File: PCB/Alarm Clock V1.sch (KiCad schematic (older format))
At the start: 23 parts, among them P1 CONN_01X02, P4 CONN_02X25, P5 CONN_02X25, SW1 SW_PUSH, SW2 SW_PUSH, SW3 SW_PUSH, SW4 SW_PUSH, SW5 SW_PUSH

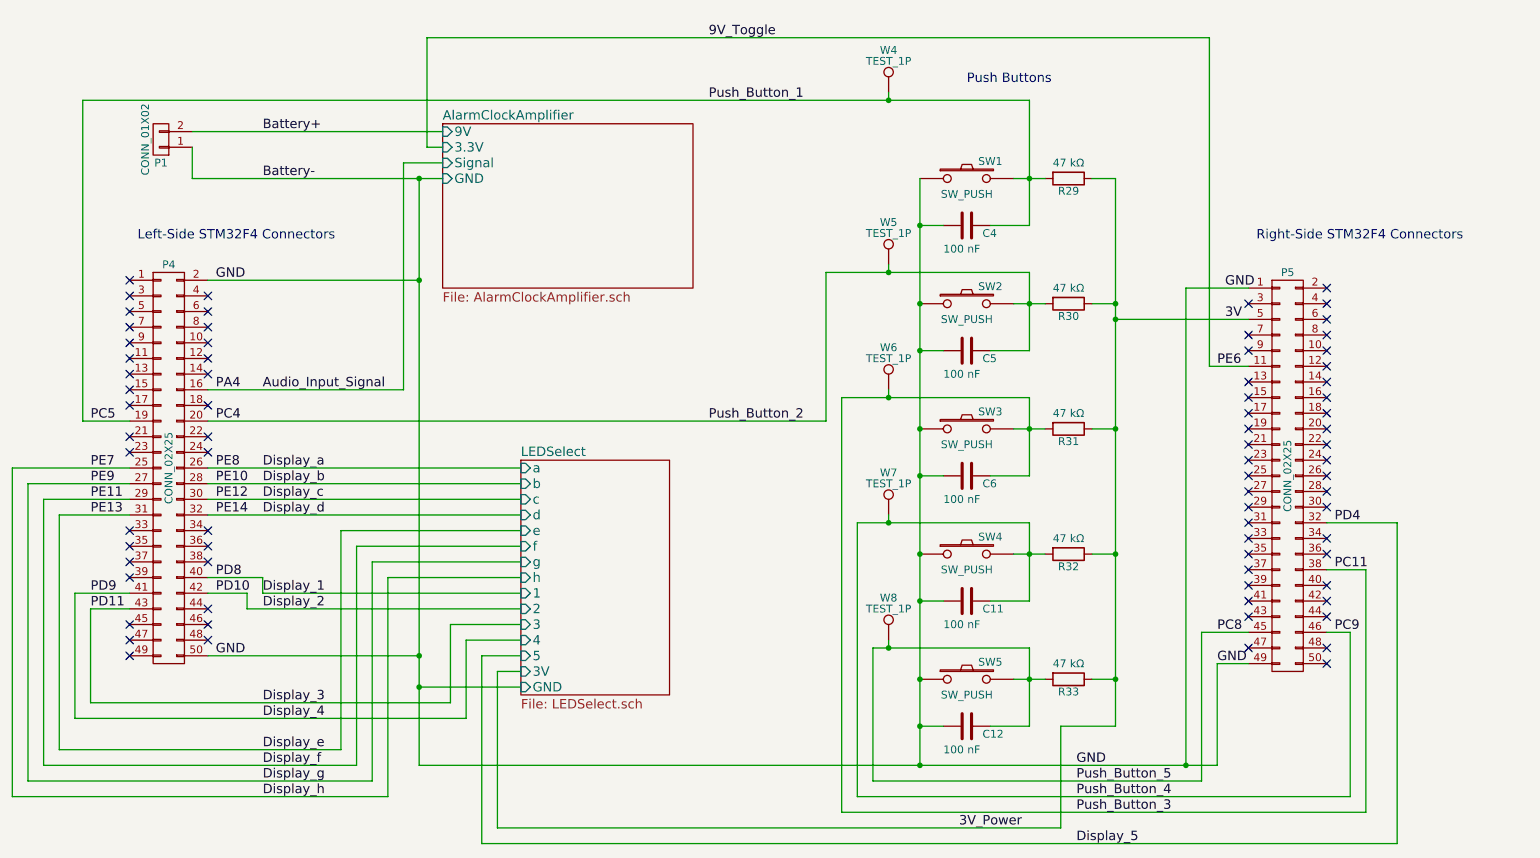
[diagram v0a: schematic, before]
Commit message: Updated PCB - Final version that was sent to fab
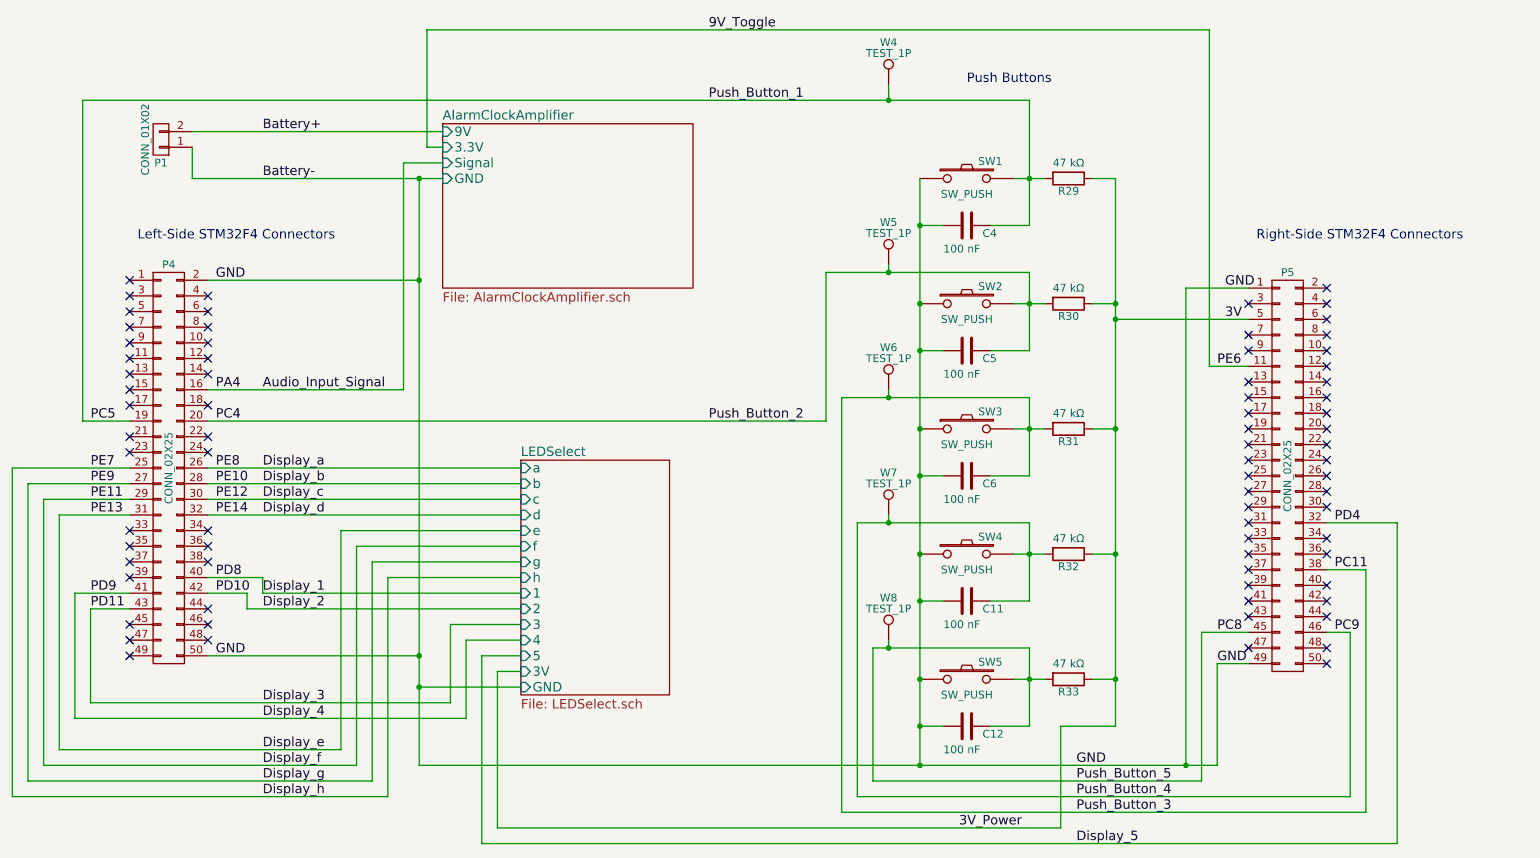
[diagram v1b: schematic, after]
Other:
- moved on the sheet: W4
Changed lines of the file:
@@
 L TEST_1P W4
 U 1 1 576C7063
-P 6200 1300
-F 0 "W4" H 6200 1570 50  0000 C CNN
-F 1 "TEST_1P" H 6200 1500 50  0000 C CNN
-F 2 "Pin_Headers:Pin_Header_Straight_1x01" H 6400 1300 50  0001 C CNN
-F 3 "" H 6400 1300 50  0000 C CNN
-	1    6200 1300
+P 6200 1250
+F 0 "W4" H 6200 1520 50  0000 C CNN
+F 1 "TEST_1P" H 6200 1450 50  0000 C CNN
+F 2 "Pin_Headers:Pin_Header_Straight_1x01" H 6400 1250 50  0001 C CNN
+F 3 "" H 6400 1250 50  0000 C CNN
+	1    6200 1250
 	1    0    0    -1
 $EndComp
@@
 Text Label 7400 5600 0    60   ~ 0
 GND
-Text Label 5050 950  0    60   ~ 0
+Text Label 5050 900  0    60   ~ 0
 9V_Toggle
 Text Label 7400 5700 0    60   ~ 0
@@
 	7100 2950 6850 2950
 Wire Wire Line
-	7100 2450 7100 2650
-Wire Wire Line
-	7100 2650 7100 2950
-Wire Wire Line
-	7000 2650 7100 2650
-Wire Wire Line
-	7100 2650 7200 2650
+	7100 2450 7100 2950
+Wire Wire Line
+	7000 2650 7200 2650
 Connection ~ 7100 2650
 Wire Wire Line
@@
 	7100 2150 6850 2150
 Wire Wire Line
-	7100 1350 7100 1850
-Wire Wire Line
-	7100 1850 7100 2150
-Wire Wire Line
-	7000 1850 7100 1850
-Wire Wire Line
-	7100 1850 7200 1850
+	7100 1350 7100 2150
+Wire Wire Line
+	7000 1850 7200 1850
 Connection ~ 7100 1850
 Wire Wire Line
@@
 	7100 4550 6850 4550
 Wire Wire Line
-	7100 4050 7100 4250
-Wire Wire Line
-	7100 4250 7100 4550
-Wire Wire Line
-	7000 4250 7100 4250
-Wire Wire Line
-	7100 4250 7200 4250
+	7100 4050 7100 4550
+Wire Wire Line
+	7000 4250 7200 4250
 Connection ~ 7100 4250
 Wire Wire Line
 	6400 4550 6550 4550
 Wire Wire Line
-	6000 4050 6200 4050
-Wire Wire Line
-	6200 4050 7100 4050
+	6000 4050 7100 4050
 Wire Wire Line
 	7100 3750 6850 3750
 Wire Wire Line
-	7100 3250 7100 3450
-Wire Wire Line
-	7100 3450 7100 3750
-Wire Wire Line
-	7000 3450 7100 3450
-Wire Wire Line
-	7100 3450 7200 3450
+	7100 3250 7100 3750
+Wire Wire Line
+	7000 3450 7200 3450
 Connection ~ 7100 3450
 Wire Wire Line
 	6400 3750 6550 3750
 Wire Wire Line
-	5900 3250 6200 3250
-Wire Wire Line
-	6200 3250 7100 3250
+	5900 3250 7100 3250
 Wire Wire Line
 	7100 5350 6850 5350
 Wire Wire Line
-	7100 4850 7100 5050
-Wire Wire Line
-	7100 5050 7100 5350
-Wire Wire Line
-	7000 5050 7100 5050
-Wire Wire Line
-	7100 5050 7200 5050
+	7100 4850 7100 5350
+Wire Wire Line
+	7000 5050 7200 5050
 Connection ~ 7100 5050
 Wire Wire Line
 	6400 5350 6550 5350
 Wire Wire Line
-	6100 4850 6200 4850
-Wire Wire Line
-	6200 4850 7100 4850
+	6100 4850 7100 4850
 Connection ~ 6400 5350
 Connection ~ 6400 4550
@@
 	3200 5100 3850 5100
 Wire Wire Line
-	6400 1850 6400 2150
-Wire Wire Line
-	6400 2150 6400 2650
-Wire Wire Line
-	6400 2650 6400 2950
-Wire Wire Line
-	6400 2950 6400 3450
-Wire Wire Line
-	6400 3450 6400 3750
-Wire Wire Line
-	6400 3750 6400 4250
-Wire Wire Line
-	6400 4250 6400 4550
-Wire Wire Line
-	6400 4550 6400 5050
-Wire Wire Line
-	6400 5050 6400 5350
-Wire Wire Line
-	6400 5350 6400 5600
+	6400 1850 6400 5600
 Wire Wire Line
 	9150 4750 9000 4750
@@
 	8200 4750 8500 4750
 Wire Wire Line
-	3200 5600 6400 5600
-Wire Wire Line
-	6400 5600 8100 5600
-Wire Wire Line
-	8100 5600 8300 5600
+	3200 5600 8300 5600
 Wire Wire Line
 	8300 5600 8300 4950
@@
 	1850 3400 5800 3400
 Wire Wire Line
-	1050 1350 6200 1350
-Wire Wire Line
-	6200 1350 7100 1350
+	1050 1350 7100 1350
 Wire Wire Line
 	1050 3400 1350 3400
 Wire Wire Line
-	1750 1850 3200 1850
-Wire Wire Line
-	3200 1850 3350 1850
+	1750 1850 3350 1850
 Wire Wire Line
 	1850 3200 3100 3200
@@
 	5800 3400 5800 2450
 Wire Wire Line
-	5800 2450 6200 2450
-Wire Wire Line
-	6200 2450 7100 2450
+	5800 2450 7100 2450
 Wire Wire Line
 	3100 3200 3100 1750
 Wire Wire Line
 	3100 1750 3350 1750
+Wire Wire Line
+	6200 1250 6200 1350
 Connection ~ 6200 1350
 Wire Wire Line
-	7650 1850 7650 2650
-Wire Wire Line
-	7650 2650 7650 2750
-Wire Wire Line
-	7650 2750 7650 3450
-Wire Wire Line
-	7650 3450 7650 4250
-Wire Wire Line
-	7650 4250 7650 5050
-Wire Wire Line
-	7650 5050 7650 5350
+	7650 1850 7650 5350
 Wire Wire Line
 	3700 5000 3850 5000
@@
 	3250 1650 3350 1650
 Wire Wire Line
+	3250 1650 3250 900
+Wire Wire Line
+	3250 900  8250 900
+Wire Wire Line
 	8250 3050 8500 3050
 Wire Wire Line
 	1750 1850 1750 1650
 Wire Wire Line
-	3200 1850 3200 2500
-Wire Wire Line
-	3200 2500 3200 4900
-Wire Wire Line
-	3200 4900 3200 5100
-Wire Wire Line
-	3200 5100 3200 5600
+	3200 1850 3200 5600
 Connection ~ 3200 1850
 Wire Wire Line
@@
 Wire Wire Line
 	1000 5300 1000 4500
+Wire Wire Line
+	8250 900  8250 3050
 Wire Wire Line
 	6100 5700 8200 5700
@@
 Connection ~ 7650 5050
 NoConn ~ 9000 2750
-Wire Wire Line
-	6200 1350 6200 1300
-Wire Wire Line
-	3250 1650 3250 950
-Wire Wire Line
-	3250 950  8250 950
-Wire Wire Line
-	8250 950  8250 3050
 $EndSCHEMATC
